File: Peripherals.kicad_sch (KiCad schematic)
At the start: 3 parts, among them J2 Conn_01x16_Socket, J3 Conn_01x16_Socket, J4 Conn_PIC_ICSP_ICD

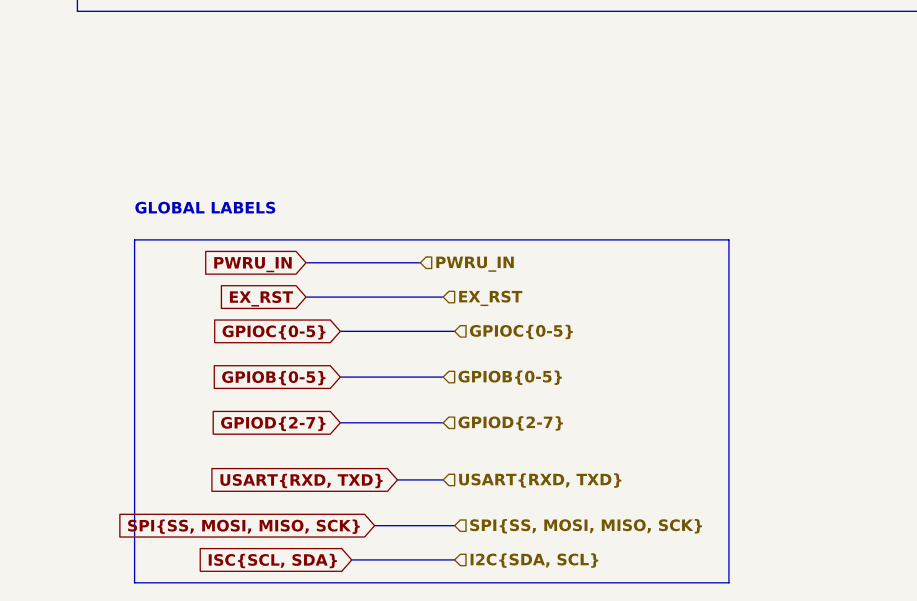
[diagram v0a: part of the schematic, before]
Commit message: updated
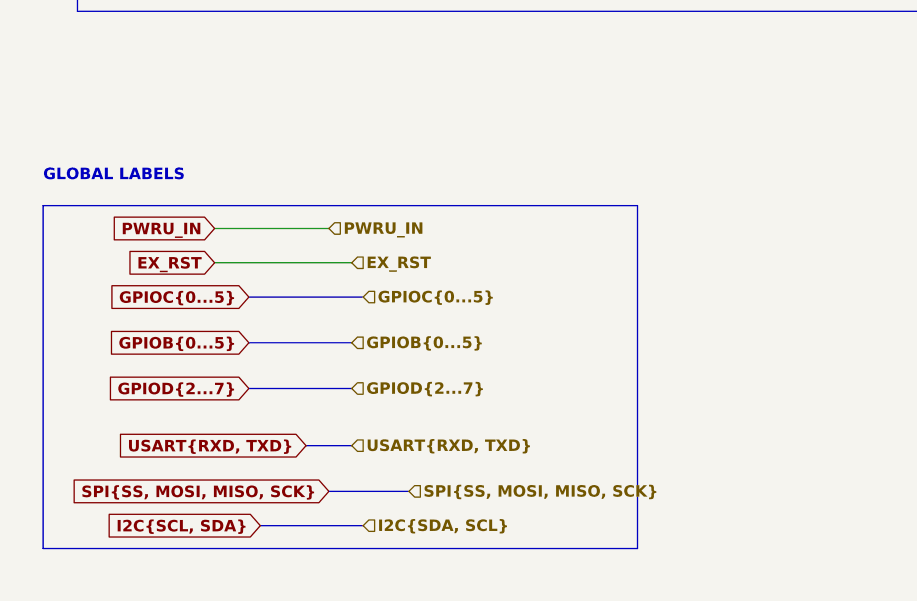
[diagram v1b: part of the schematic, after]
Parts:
- J2, J3: footprint (none) -> Connector_PinHeader_2.54mm:PinHeader_1x16_P2.54mm_Vertical
- J4: footprint (none) -> Connector_PinSocket_2.54mm:PinSocket_2x03_P2.54mm_Vertical
